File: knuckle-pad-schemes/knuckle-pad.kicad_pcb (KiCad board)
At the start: 2 copper layers, 128.5 x 116.2 mm, 66 parts, among them SW1 SW_Push, SW10 SW_Push, SW11 SW_Push, SW12 SW_Push, SW13 SW_Push, SW14 SW_Push, SW15 SW_Push, SW16 SW_Push, SW17 SW_Push, SW18 SW_Push, SW19 SW_Push, SW2 SW_Push, SW20 SW_Push, SW21 SW_Push, SW22 SW_Push, SW23 SW_Push, SW24 SW_Push, SW25 SW_Push, SW26 SW_Push, SW27 SW_Push, SW28 SW_Push, SW29 SW_Push, SW3 SW_Push, SW4 SW_Push, SW5 SW_Push, SW6 SW_Push, SW7 SW_Push, SW8 SW_Push, SW9 SW_Push, U1 ProMicro

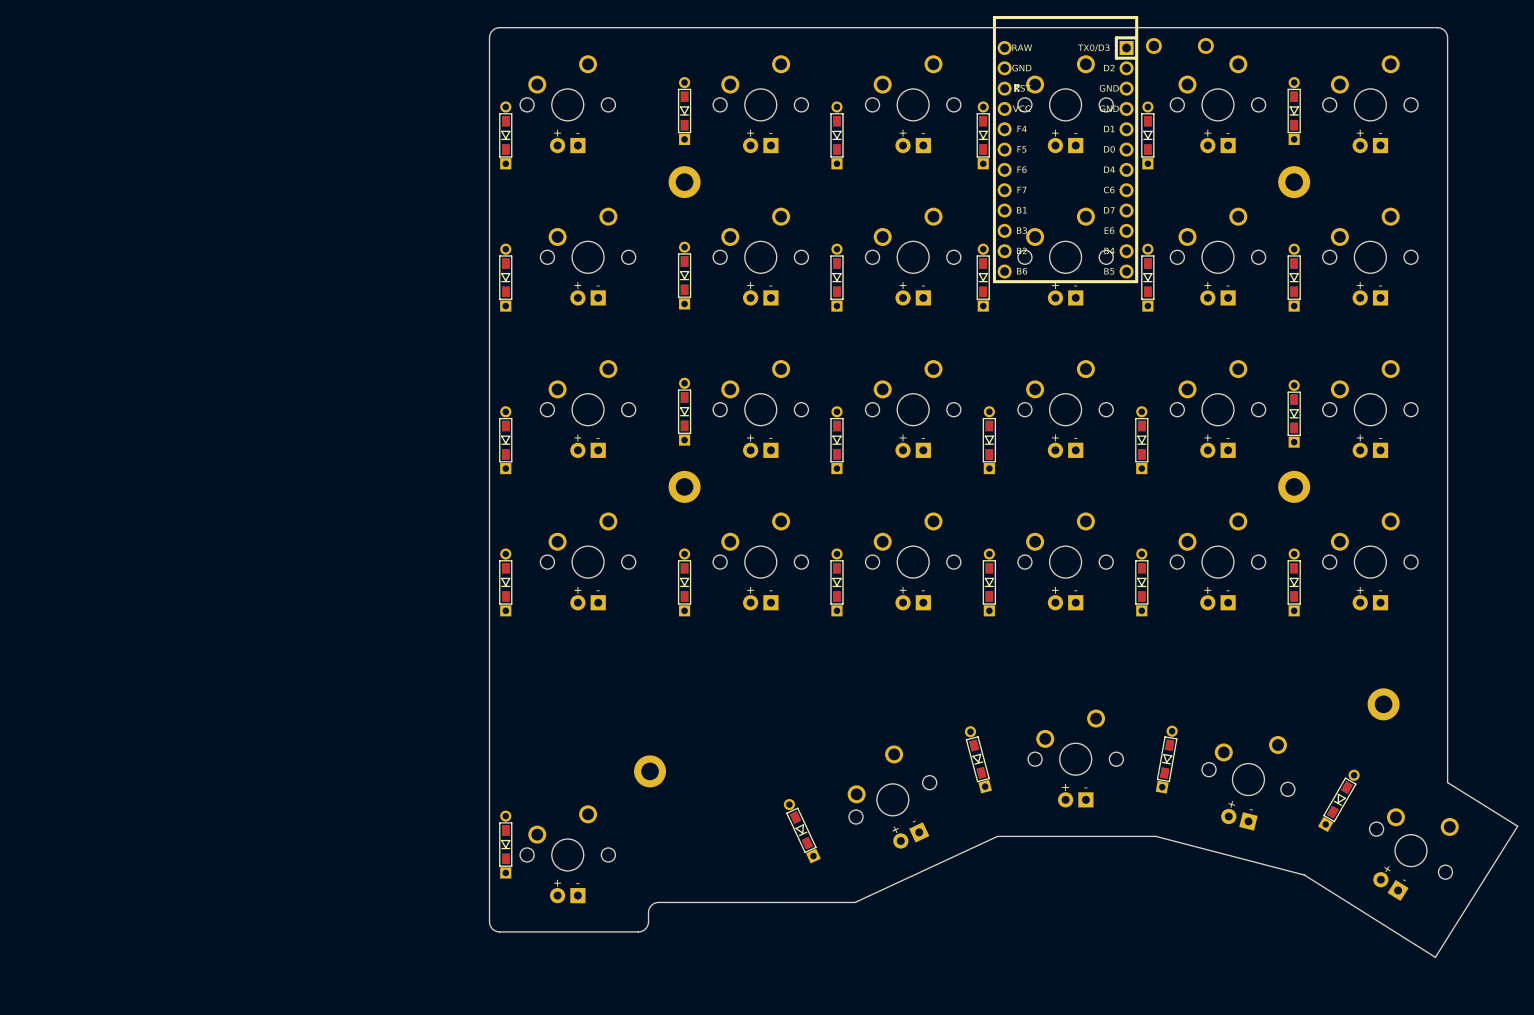
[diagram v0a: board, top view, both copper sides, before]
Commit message: rounded all edges(
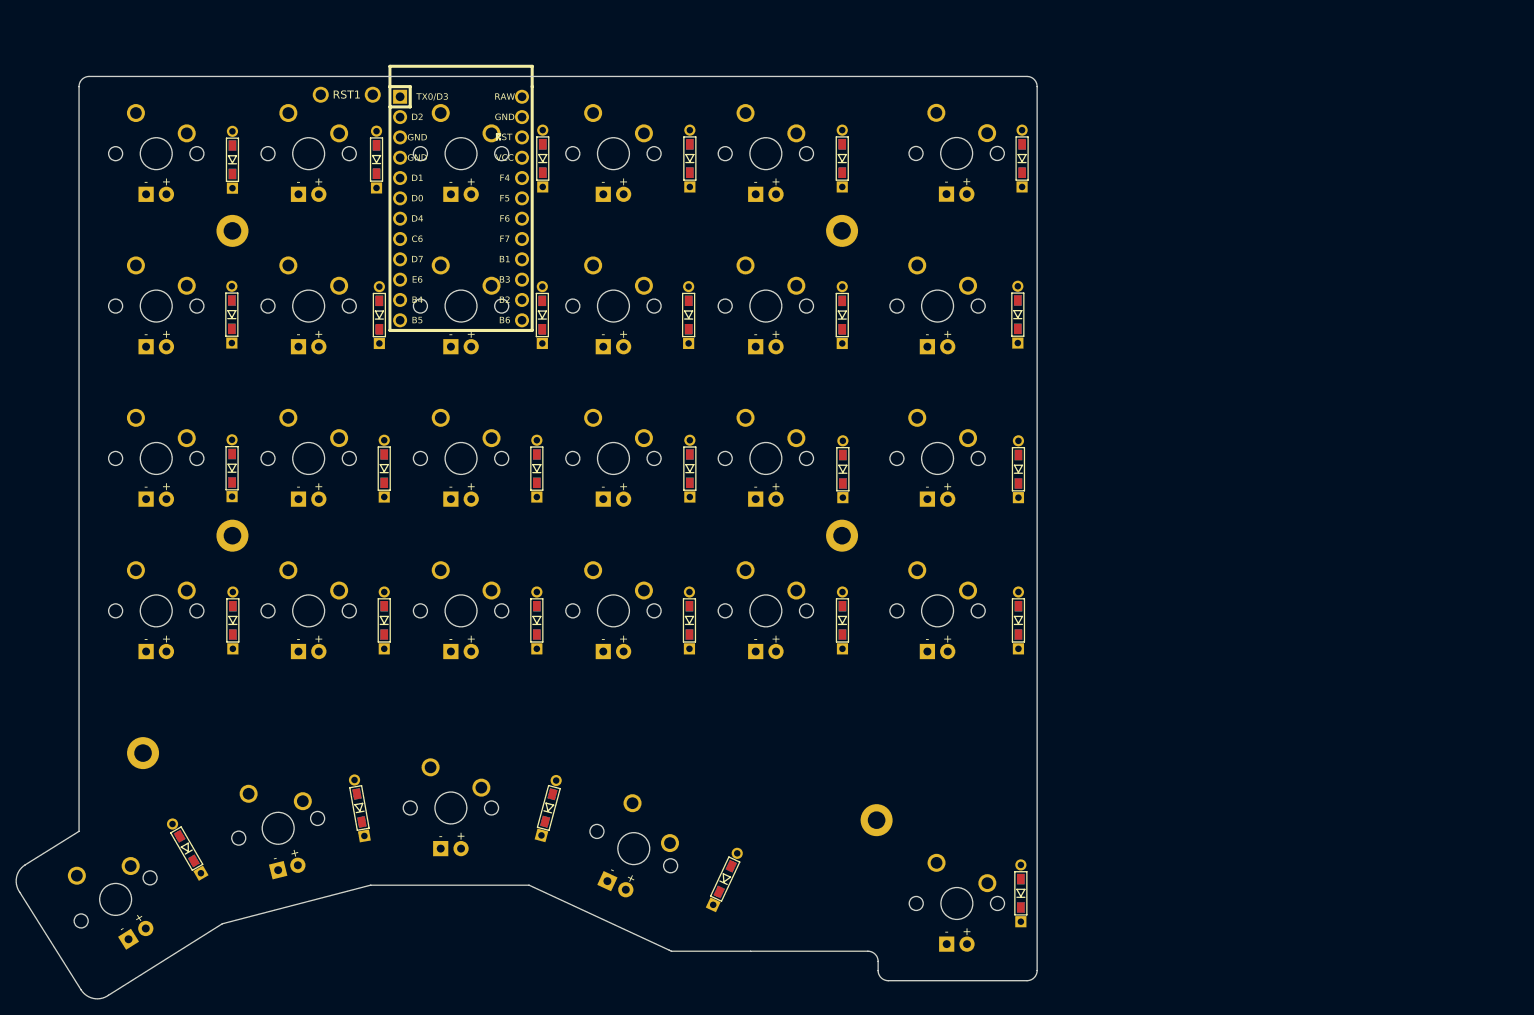
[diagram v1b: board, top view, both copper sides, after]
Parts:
- D1, D10, D11, D12, D13, D14, D15, D16, D17, D18, D19, D2, D20, D21, D22, D23, D24, D25, D26, D27, D28, D29, D3, D4, D5, D6, D7, D8, D9, RST1, U1: moved to F.Cu
- H1, H2, H3, H4, H5, H6, SW1, SW10, SW11, SW12, SW13, SW14, SW15, SW16, SW17, SW18, SW19, SW2, SW20, SW21, SW22, SW23, SW24, SW25, SW26, SW27, SW28, SW29, SW3, SW4, SW5, SW6, SW7, SW8, SW9: moved to B.Cu
- moved SW29 162.0 mm to (105.4, 126.0), turned to 212 degrees
- moved H6 155.2 mm to (108.8, 107.7), turned to 180 degrees
- moved SW25 151.9 mm to (110.5, 32.8), turned to 180 degrees
- moved SW26 151.9 mm to (110.5, 51.8), turned to 180 degrees
- moved SW27 151.9 mm to (110.5, 70.9), turned to 180 degrees
- moved SW28 151.9 mm to (110.5, 89.9), turned to 180 degrees
- moved D29 144.3 mm to (114.3, 119.6), turned to 120 degrees
- moved D27 132.9 mm to (120.0, 72.1)
- moved D26 132.9 mm to (119.9, 52.9)
- moved D25 132.9 mm to (120.0, 33.5)
- moved H1 132.9 mm to (120.0, 80.5), turned to 180 degrees
- moved H5 132.9 mm to (120.0, 42.4), turned to 180 degrees
- moved D28 132.7 mm to (120.1, 91.1)
- moved SW24 121.4 mm to (125.7, 117.1), turned to 194 degrees
- moved SW20 113.8 mm to (129.5, 32.8), turned to 180 degrees
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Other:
- board size 128.5 x 116.2 mm -> 127.6 x 115.3 mm
